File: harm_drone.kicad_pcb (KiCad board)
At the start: 2 copper layers, 90 x 40 mm, 0 parts

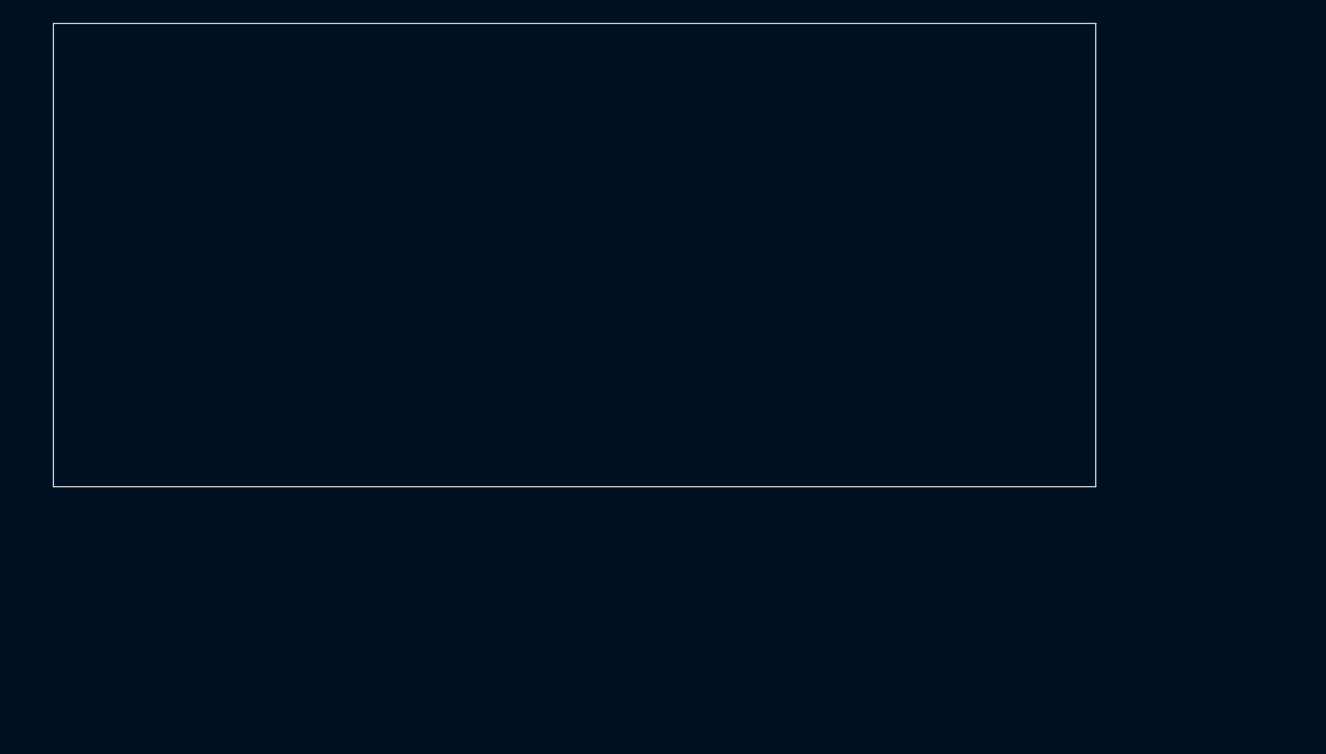
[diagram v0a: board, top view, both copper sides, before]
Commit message: initial PCB draft!
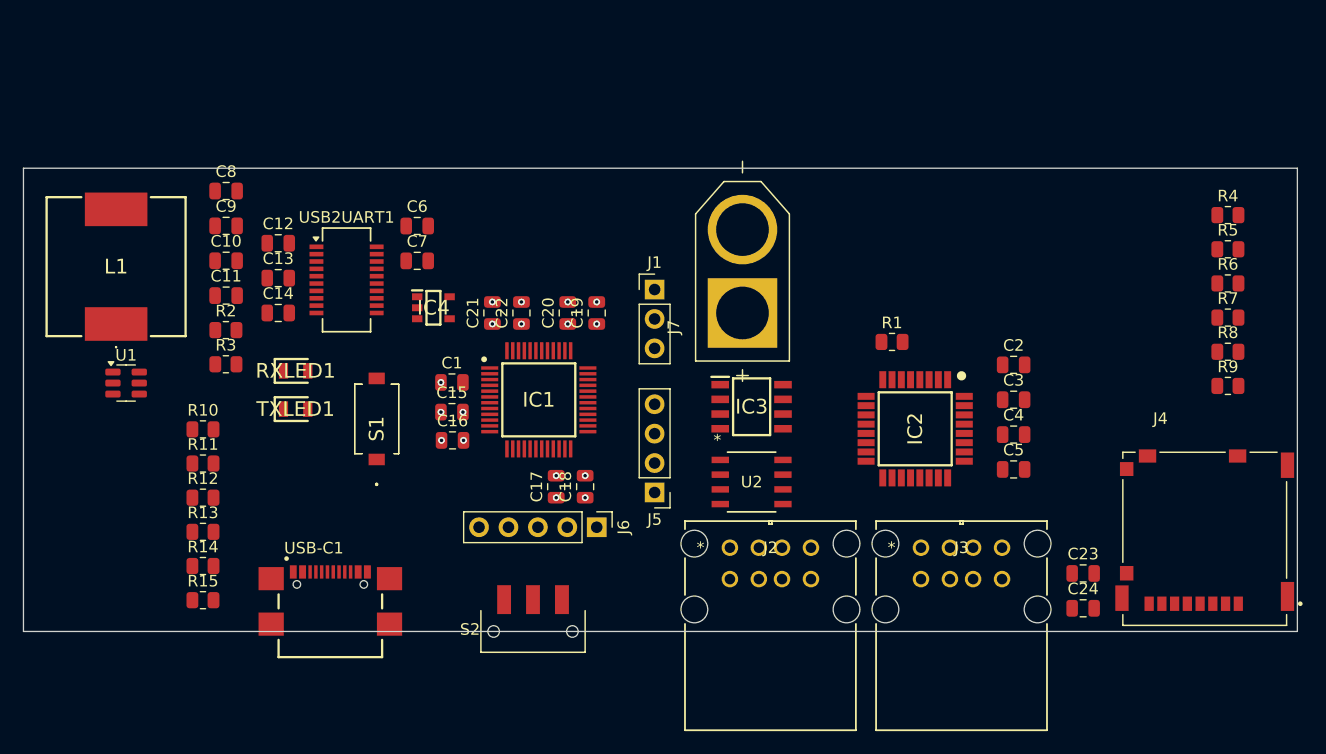
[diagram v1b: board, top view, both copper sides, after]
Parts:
- added C1: 0.1uF, Capacitor_SMD:C_0805_2012Metric, F.Cu at (131.9, 96.5)
- added C10: 22uF, Capacitor_SMD:C_0805_2012Metric, F.Cu at (112.4, 86.0)
- added C11: 22uF, Capacitor_SMD:C_0805_2012Metric, F.Cu at (112.4, 89.0)
- added C12: 47pF, Capacitor_SMD:C_0805_2012Metric, F.Cu at (116.9, 84.5)
- added C13: 47pF, Capacitor_SMD:C_0805_2012Metric, F.Cu at (116.9, 87.5)
- added C14: 1uF, Capacitor_SMD:C_0805_2012Metric, F.Cu at (116.9, 90.5)
- added C15: 10uF, Capacitor_SMD:C_0805_2012Metric, F.Cu at (131.9, 99.1)
- added C16: 0.1uF, Capacitor_SMD:C_0805_2012Metric, F.Cu at (132.0, 101.5)
- added C17: 0.1uF, Capacitor_SMD:C_0805_2012Metric, F.Cu at (140.9, 105.5)
- added C18: 10uF, Capacitor_SMD:C_0805_2012Metric, F.Cu at (143.4, 105.5)
- added C19: 10uF, Capacitor_SMD:C_0805_2012Metric, F.Cu at (144.4, 90.5)
- added C2: 10uF, Capacitor_SMD:C_0805_2012Metric, F.Cu at (180.4, 95.0)
- added C20: 0.1uF, Capacitor_SMD:C_0805_2012Metric, F.Cu at (141.9, 90.5)
- added C21: 10uF, Capacitor_SMD:C_0805_2012Metric, F.Cu at (135.4, 90.5)
- added C22: 0.1uF, Capacitor_SMD:C_0805_2012Metric, F.Cu at (137.9, 90.5)
- added C23: 10uF, Capacitor_SMD:C_0805_2012Metric, F.Cu at (186.4, 113.0)
- added C24: 0.1uF, Capacitor_SMD:C_0805_2012Metric, F.Cu at (186.4, 116.0)
- added C3: 0.1uF, Capacitor_SMD:C_0805_2012Metric, F.Cu at (180.4, 98.0)
- added C4: 0.1uF, Capacitor_SMD:C_0805_2012Metric, F.Cu at (180.4, 101.0)
- added C5: 10uF, Capacitor_SMD:C_0805_2012Metric, F.Cu at (180.4, 104.0)
- added C6: 1uF, Capacitor_SMD:C_0805_2012Metric, F.Cu at (128.9, 83.0)
- added C7: 1uF, Capacitor_SMD:C_0805_2012Metric, F.Cu at (128.9, 86.0)
- added C8: 0.1uFCap, Capacitor_SMD:C_0805_2012Metric, F.Cu at (112.4, 80.0)
- added C9: 0.1uF, Capacitor_SMD:C_0805_2012Metric, F.Cu at (112.4, 83.0)
- added IC1: Microcontroller, group127:Microcontroller, F.Cu at (139.4, 98.0)
- added IC2: USB Hub, group127:USB-HUB, F.Cu at (171.9, 100.5)
- added IC3: SRAM, group127:SRAM, F.Cu at (157.8, 98.6)
- added IC4: LDO, group127:LDO, F.Cu at (130.3, 90.0)
- added J1: SYS_DEBUG, Connector_PinHeader_2.54mm:PinHeader_1x03_P2.54mm_Vertical, F.Cu at (149.4, 88.5)
- added J2: 2-Port USB, group127:USBPorts, F.Cu at (155.9, 110.8)
- added J3: 2-Port USB, group127:USBPorts, F.Cu at (172.4, 110.8)
- added J4: SD_Card, group127:SDCard, F.Cu at (196.9, 110.0)
- added J5: SPI2, Connector_PinHeader_2.54mm:PinHeader_1x04_P2.54mm_Vertical, F.Cu at (149.4, 106.0)
- added J6: SPI1, Connector_PinHeader_2.54mm:PinHeader_1x05_P2.54mm_Vertical, F.Cu at (144.4, 109.0)
- added J7: XT60-M, group127:XT60-M, F.Cu at (157.0, 86.9)
- added L1: 6.8uH, group127:Inductor, F.Cu at (102.9, 86.5)
- added R1: 2kOhm, Resistor_SMD:R_0805_2012Metric, F.Cu at (169.9, 93.0)
- added R10: 27ohm, Resistor_SMD:R_0805_2012Metric, F.Cu at (110.4, 100.5)
- added R11: 27ohm, Resistor_SMD:R_0805_2012Metric, F.Cu at (110.4, 103.5)
- added R12: 270ohm, Resistor_SMD:R_0805_2012Metric, F.Cu at (110.4, 106.5)
- added R13: 270ohm, Resistor_SMD:R_0805_2012Metric, F.Cu at (110.4, 109.4)
- added R14: 5.1kohm, Resistor_SMD:R_0805_2012Metric, F.Cu at (110.4, 112.3)
- added R15: 5.1kohm, Resistor_SMD:R_0805_2012Metric, F.Cu at (110.4, 115.3)
- added R2: 100k, Resistor_SMD:R_0805_2012Metric, F.Cu at (112.4, 92.0)
- added R3: 13.7k, Resistor_SMD:R_0805_2012Metric, F.Cu at (112.4, 94.9)
- added R4: 10kOhm, Resistor_SMD:R_0805_2012Metric, F.Cu at (198.9, 82.0)
- added R5: 10kOhm, Resistor_SMD:R_0805_2012Metric, F.Cu at (198.9, 85.0)
- added R6: 27, Resistor_SMD:R_0805_2012Metric, F.Cu at (198.9, 88.0)
- added R7: 10kOhm, Resistor_SMD:R_0805_2012Metric, F.Cu at (198.9, 90.9)
- added R8: 10kOhm, Resistor_SMD:R_0805_2012Metric, F.Cu at (198.9, 93.8)
- added R9: 10kOhm, Resistor_SMD:R_0805_2012Metric, F.Cu at (198.9, 96.8)
- added RXLED1: SM0805UBWC, KiCad0805:LEDC2012X110N, F.Cu at (118.4, 95.5)
- added S1: KSR221GLFS, group127:Button, F.Cu at (125.4, 99.7)
- added S2: Switch, JS102011SAQN:SW_JS102011SAQN, F.Cu at (138.9, 118.0)
- added TXLED1: SM0805UBWC, KiCad0805:LEDC2012X110N, F.Cu at (118.4, 98.8)
- added U1: LMR51430, Package_TO_SOT_SMD:SOT-23-6, F.Cu at (103.8, 96.5)
- added U2: EEPROM, group127:EEPROM, F.Cu at (157.8, 105.1)
- added USB-C1: USB4110GFA, USB4110_GF_A:GCT_USB4110GFA, F.Cu at (121.4, 113.9)
- added USB2UART1: FT231XS-R, Package_SO:SSOP-20_3.9x8.7mm_P0.635mm, F.Cu at (122.8, 87.6)
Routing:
- net GND: vias 0 -> 9
- net 3V3: vias 0 -> 8
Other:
- board size 90 x 40 mm -> 110 x 40 mm
- copper layers 2 -> 4
